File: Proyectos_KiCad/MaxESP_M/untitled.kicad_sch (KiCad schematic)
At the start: 30 parts, among them J3 PJ-325M/3.5MM, J4 DA15, J5 Conn_01x04, J6 RJ12, J9 RTC, U4 WEMOS_C3_mini

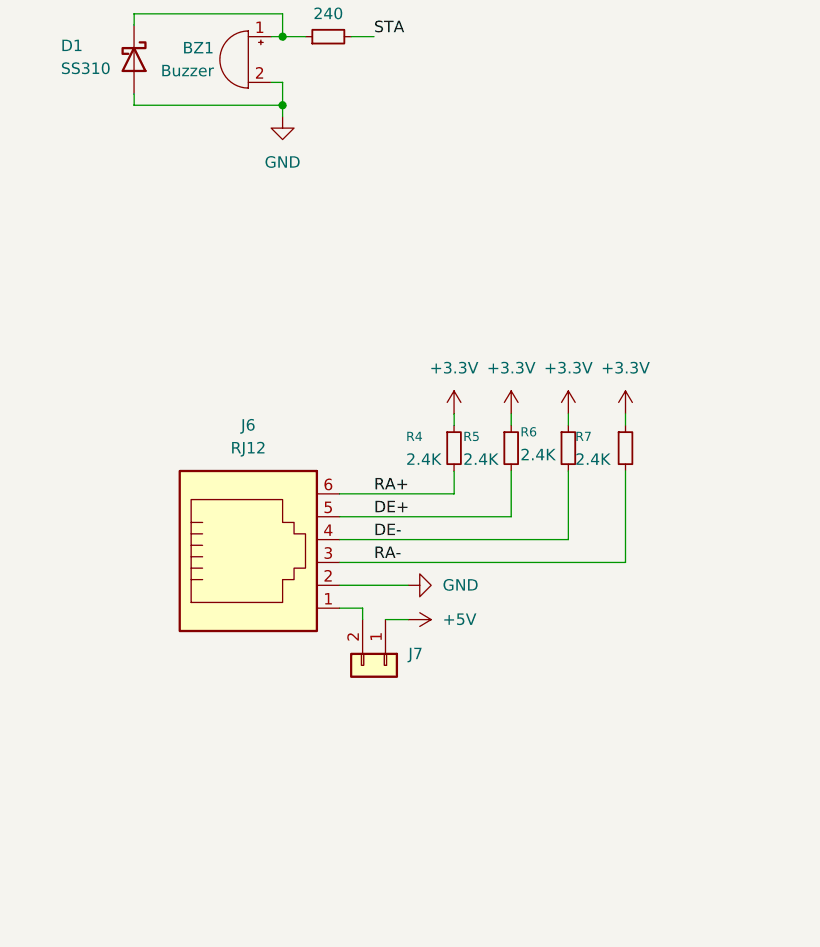
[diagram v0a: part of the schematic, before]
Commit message: Por si valgo
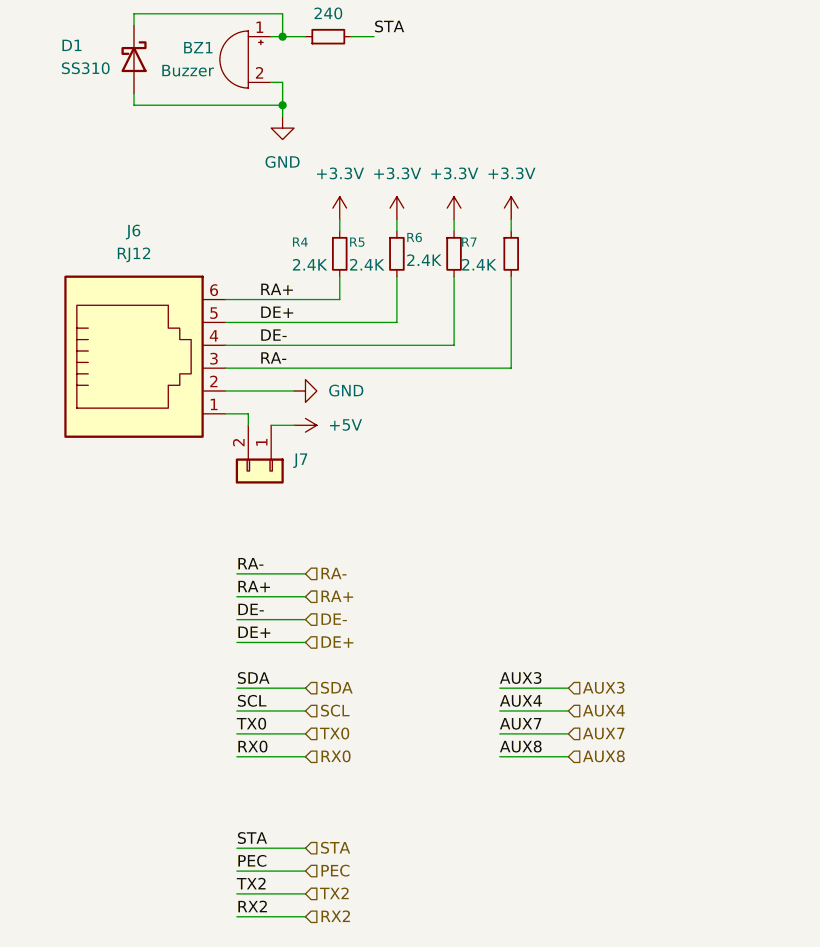
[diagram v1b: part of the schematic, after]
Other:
- moved on the sheet: J6, J7, R4, R5, R6, R7
